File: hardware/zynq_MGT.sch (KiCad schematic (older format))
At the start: 6 parts, among them U201 xc7z030sbg485

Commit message: Fixed Schematic Symbols
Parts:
- C1001, C1002, C1003, C1004: symbol device:C_Small -> Device:C_Small
- R1001: symbol device:R_Small -> Device:R_Small
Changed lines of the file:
@@
 $Descr A4 11693 8268
 encoding utf-8
-Sheet 10 22
+Sheet 10 21
 Title ""
 Date ""
@@
 MGTREFCLK_1_P
 $Comp
-L device:C_Small C1004
+L Device:C_Small C1004
 U 1 1 598A74A2
 P 4250 2550
@@
 $EndComp
 $Comp
-L device:C_Small C1003
+L Device:C_Small C1003
 U 1 1 598A7543
 P 4000 2450
@@
 $EndComp
 $Comp
-L device:C_Small C1001
+L Device:C_Small C1001
 U 1 1 598A7566
 P 3500 2250
@@
 $EndComp
 $Comp
-L device:C_Small C1002
+L Device:C_Small C1002
 U 1 1 598A75B1
 P 3750 2350
@@
 MGTX_TX_0_P
 $Comp
-L device:R_Small R1001
+L Device:R_Small R1001
 U 1 1 5ADF6841
 P 5100 2150

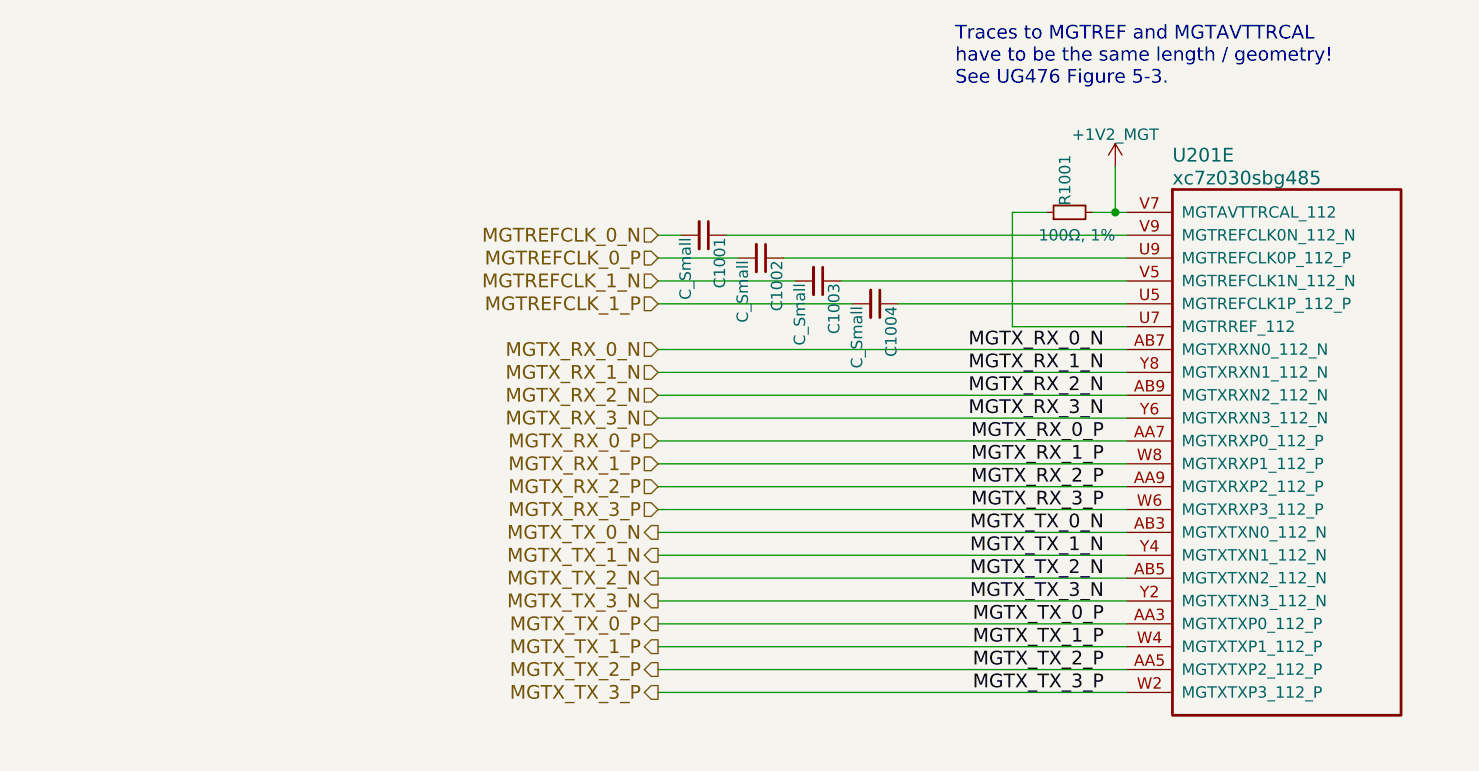
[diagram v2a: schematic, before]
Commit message: Xaui lanes
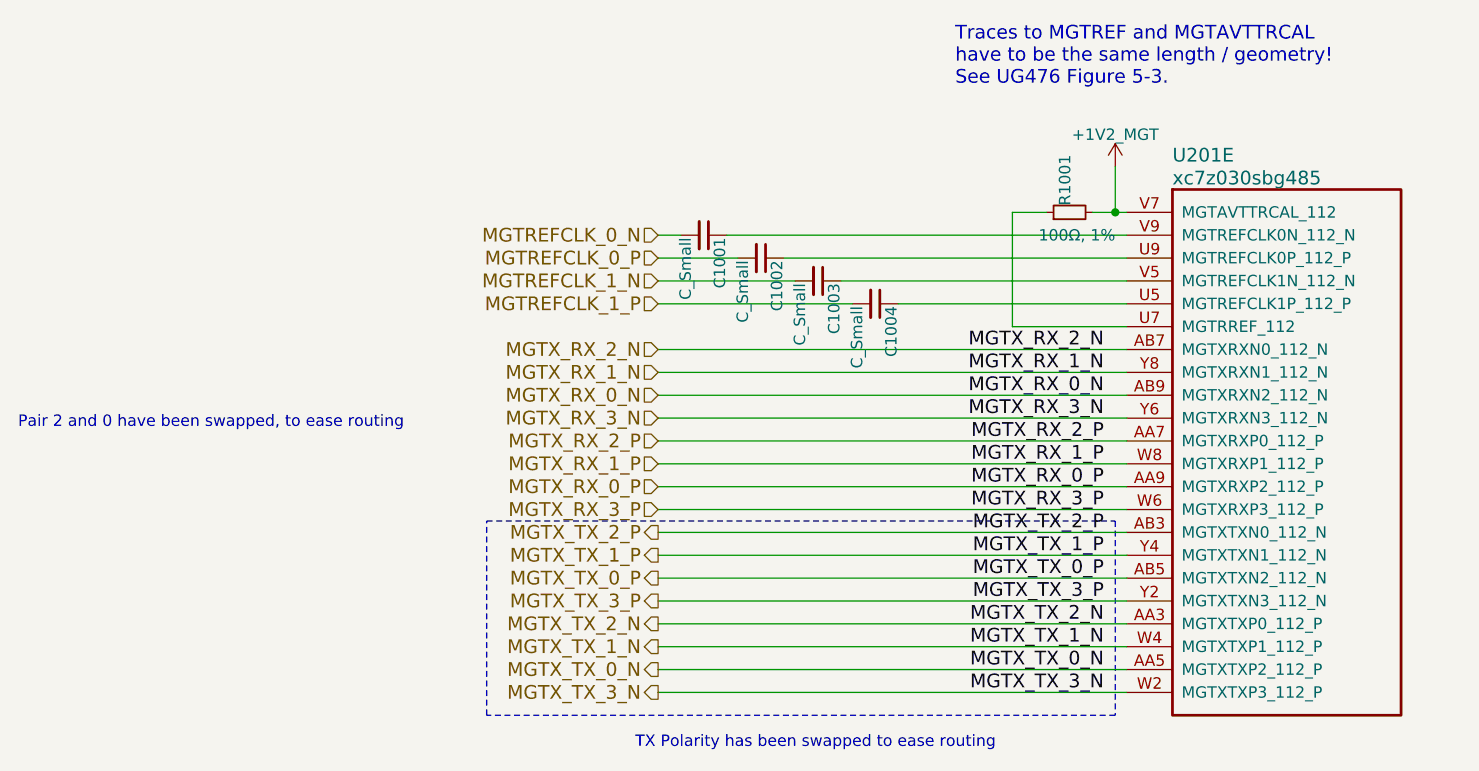
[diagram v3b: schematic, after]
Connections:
- net MGTX_RX_0_N: now also U201.AB9 (MGTXRXN2_112_N); no longer U201.AB7 (MGTXRXN0_112_N)
- net MGTX_RX_0_P: now also U201.AA9 (MGTXRXP2_112_P); no longer U201.AA7 (MGTXRXP0_112_P)
- net MGTX_RX_2_N: now also U201.AB7 (MGTXRXN0_112_N); no longer U201.AB9 (MGTXRXN2_112_N)
- net MGTX_RX_2_P: now also U201.AA7 (MGTXRXP0_112_P); no longer U201.AA9 (MGTXRXP2_112_P)
- net MGTX_TX_0_N: now also U201.AA5 (MGTXTXP2_112_P); no longer U201.AB3 (MGTXTXN0_112_N)
- net MGTX_TX_0_P: now also U201.AB5 (MGTXTXN2_112_N); no longer U201.AA3 (MGTXTXP0_112_P)
- net MGTX_TX_1_N: now also U201.W4 (MGTXTXP1_112_P); no longer U201.Y4 (MGTXTXN1_112_N)
- net MGTX_TX_1_P: now also U201.Y4 (MGTXTXN1_112_N); no longer U201.W4 (MGTXTXP1_112_P)
- net MGTX_TX_2_N: now also U201.AA3 (MGTXTXP0_112_P); no longer U201.AB5 (MGTXTXN2_112_N)
- net MGTX_TX_2_P: now also U201.AB3 (MGTXTXN0_112_N); no longer U201.AA5 (MGTXTXP2_112_P)
- net MGTX_TX_3_N: now also U201.W2 (MGTXTXP3_112_P); no longer U201.Y2 (MGTXTXN3_112_N)
- net MGTX_TX_3_P: now also U201.Y2 (MGTXTXN3_112_N); no longer U201.W2 (MGTXTXP3_112_P)
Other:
- note added: "Pair 2 and 0 have been swapped, to ease routing"
- note added: "TX Polarity has been swapped to ease routing"
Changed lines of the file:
@@
 	1    0    0    -1
 $EndComp
-Text HLabel 3300 2750 0    60   Input ~ 0
+Text HLabel 3300 2950 0    60   Input ~ 0
 MGTX_RX_0_N
 Text HLabel 3300 2850 0    60   Input ~ 0
 MGTX_RX_1_N
-Text HLabel 3300 2950 0    60   Input ~ 0
+Text HLabel 3300 2750 0    60   Input ~ 0
 MGTX_RX_2_N
 Text HLabel 3300 3050 0    60   Input ~ 0
 MGTX_RX_3_N
-Text HLabel 3300 3150 0    60   Input ~ 0
+Text HLabel 3300 3350 0    60   Input ~ 0
 MGTX_RX_0_P
 Text HLabel 3300 3250 0    60   Input ~ 0
 MGTX_RX_1_P
-Text HLabel 3300 3350 0    60   Input ~ 0
+Text HLabel 3300 3150 0    60   Input ~ 0
 MGTX_RX_2_P
 Text HLabel 3300 3450 0    60   Input ~ 0
 MGTX_RX_3_P
+Text HLabel 3300 4150 0    60   Output ~ 0
+MGTX_TX_0_N
+Text HLabel 3300 4050 0    60   Output ~ 0
+MGTX_TX_1_N
+Text HLabel 3300 3950 0    60   Output ~ 0
+MGTX_TX_2_N
+Text HLabel 3300 4250 0    60   Output ~ 0
+MGTX_TX_3_N
+Text HLabel 3300 3750 0    60   Output ~ 0
+MGTX_TX_0_P
+Text HLabel 3300 3650 0    60   Output ~ 0
+MGTX_TX_1_P
 Text HLabel 3300 3550 0    60   Output ~ 0
-MGTX_TX_0_N
-Text HLabel 3300 3650 0    60   Output ~ 0
-MGTX_TX_1_N
-Text HLabel 3300 3750 0    60   Output ~ 0
-MGTX_TX_2_N
+MGTX_TX_2_P
 Text HLabel 3300 3850 0    60   Output ~ 0
-MGTX_TX_3_N
-Text HLabel 3300 3950 0    60   Output ~ 0
-MGTX_TX_0_P
-Text HLabel 3300 4050 0    60   Output ~ 0
-MGTX_TX_1_P
-Text HLabel 3300 4150 0    60   Output ~ 0
-MGTX_TX_2_P
-Text HLabel 3300 4250 0    60   Output ~ 0
 MGTX_TX_3_P
 Text HLabel 3300 2250 0    60   Input ~ 0
@@
 	3300 2550 4150 2550
 Wire Wire Line
+	3300 2950 5350 2950
+Wire Wire Line
+	5350 2850 3300 2850
+Wire Wire Line
 	3300 2750 5350 2750
 Wire Wire Line
-	5350 2850 3300 2850
-Wire Wire Line
-	3300 2950 5350 2950
-Wire Wire Line
 	5350 3050 3300 3050
 Wire Wire Line
+	3300 3350 5350 3350
+Wire Wire Line
+	5350 3250 3300 3250
+Wire Wire Line
 	3300 3150 5350 3150
 Wire Wire Line
-	5350 3250 3300 3250
-Wire Wire Line
-	3300 3350 5350 3350
-Wire Wire Line
 	5350 3450 3300 3450
 Wire Wire Line
+	3300 4150 5350 4150
+Wire Wire Line
+	5350 4050 3300 4050
+Wire Wire Line
+	3300 3950 5350 3950
+Wire Wire Line
+	5350 4250 3300 4250
+Wire Wire Line
+	3300 3750 5350 3750
+Wire Wire Line
+	5350 3650 3300 3650
+Wire Wire Line
 	3300 3550 5350 3550
 Wire Wire Line
-	5350 3650 3300 3650
-Wire Wire Line
-	3300 3750 5350 3750
-Wire Wire Line
 	5350 3850 3300 3850
-Wire Wire Line
-	3300 3950 5350 3950
-Wire Wire Line
-	5350 4050 3300 4050
-Wire Wire Line
-	3300 4150 5350 4150
-Wire Wire Line
-	5350 4250 3300 4250
 Text Label 5250 2850 2    60   ~ 0
 MGTX_RX_1_N
-Text Label 5250 2950 2    60   ~ 0
+Text Label 5250 2750 2    60   ~ 0
 MGTX_RX_2_N
 Text Label 5250 3050 2    60   ~ 0
@@
 Text Label 5250 3250 2    60   ~ 0
 MGTX_RX_1_P
-Text Label 5250 3350 2    60   ~ 0
+Text Label 5250 3150 2    60   ~ 0
 MGTX_RX_2_P
 Text Label 5250 3450 2    60   ~ 0
 MGTX_RX_3_P
+Text Label 5250 4050 2    60   ~ 0
+MGTX_TX_1_N
+Text Label 5250 3950 2    60   ~ 0
+MGTX_TX_2_N
+Text Label 5250 4250 2    60   ~ 0
+MGTX_TX_3_N
 Text Label 5250 3650 2    60   ~ 0
-MGTX_TX_1_N
+MGTX_TX_1_P
+Text Label 5250 3550 2    60   ~ 0
+MGTX_TX_2_P
+Text Label 5250 3850 2    60   ~ 0
+MGTX_TX_3_P
+Text Label 5250 3350 2    60   ~ 0
+MGTX_RX_0_P
+Text Label 5250 2950 2    60   ~ 0
+MGTX_RX_0_N
+Text Label 5250 4150 2    60   ~ 0
+MGTX_TX_0_N
 Text Label 5250 3750 2    60   ~ 0
-MGTX_TX_2_N
-Text Label 5250 3850 2    60   ~ 0
-MGTX_TX_3_N
-Text Label 5250 4050 2    60   ~ 0
-MGTX_TX_1_P
-Text Label 5250 4150 2    60   ~ 0
-MGTX_TX_2_P
-Text Label 5250 4250 2    60   ~ 0
-MGTX_TX_3_P
-Text Label 5250 3150 2    60   ~ 0
-MGTX_RX_0_P
-Text Label 5250 2750 2    60   ~ 0
-MGTX_RX_0_N
-Text Label 5250 3550 2    60   ~ 0
-MGTX_TX_0_N
-Text Label 5250 3950 2    60   ~ 0
 MGTX_TX_0_P
 $Comp
@@
 Wire Wire Line
 	5300 2150 5350 2150
+Wire Notes Line
+	2550 3500 5300 3500
+Wire Notes Line
+	5300 3500 5300 4350
+Wire Notes Line
+	5300 4350 2550 4350
+Wire Notes Line
+	2550 4350 2550 3500
+Text Notes 3200 4500 0    50   ~ 0
+TX Polarity has been swapped to ease routing
+Text Notes 500  3100 0    50   ~ 0
+Pair 2 and 0 have been swapped, to ease routing
 $EndSCHEMATC
